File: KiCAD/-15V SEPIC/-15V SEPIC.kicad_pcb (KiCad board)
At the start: 4 copper layers, 33.8 x 28.9 mm, 16 parts, among them U1 LT3579

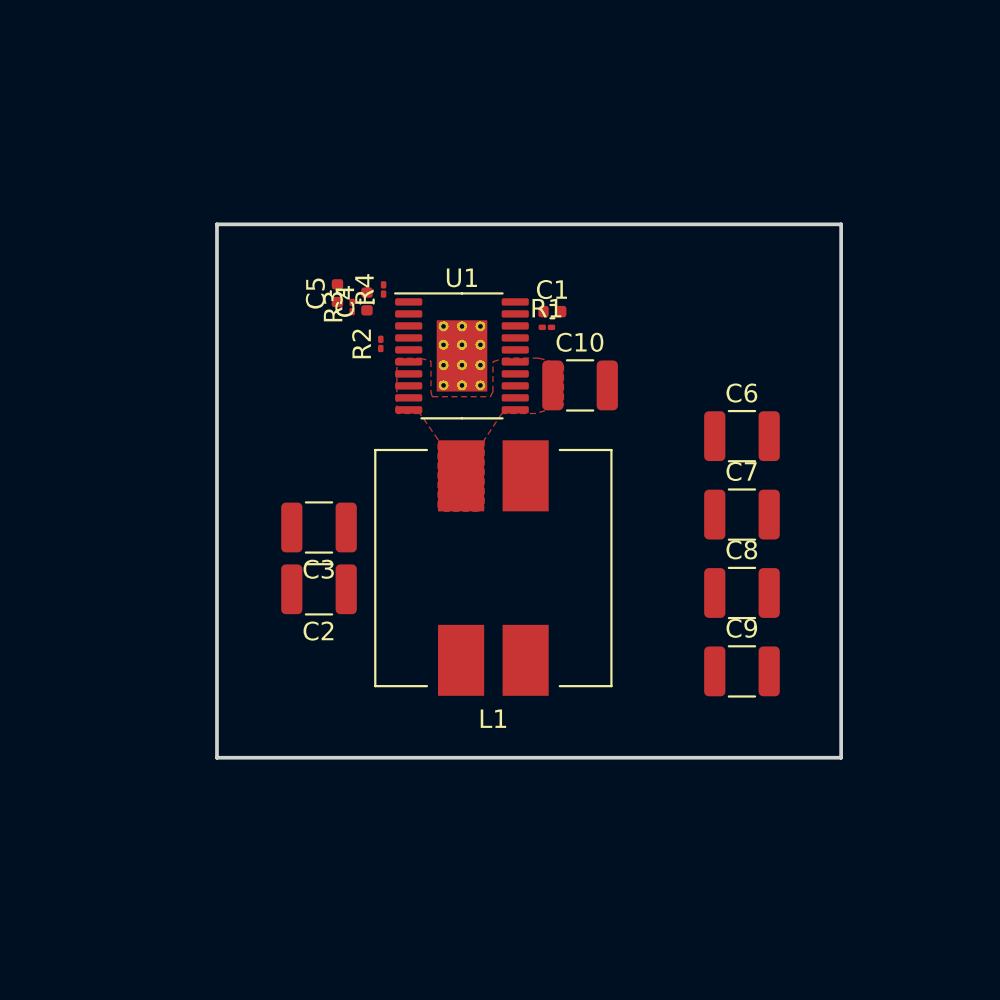
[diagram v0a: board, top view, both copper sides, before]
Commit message: work on speic schematic and PCB
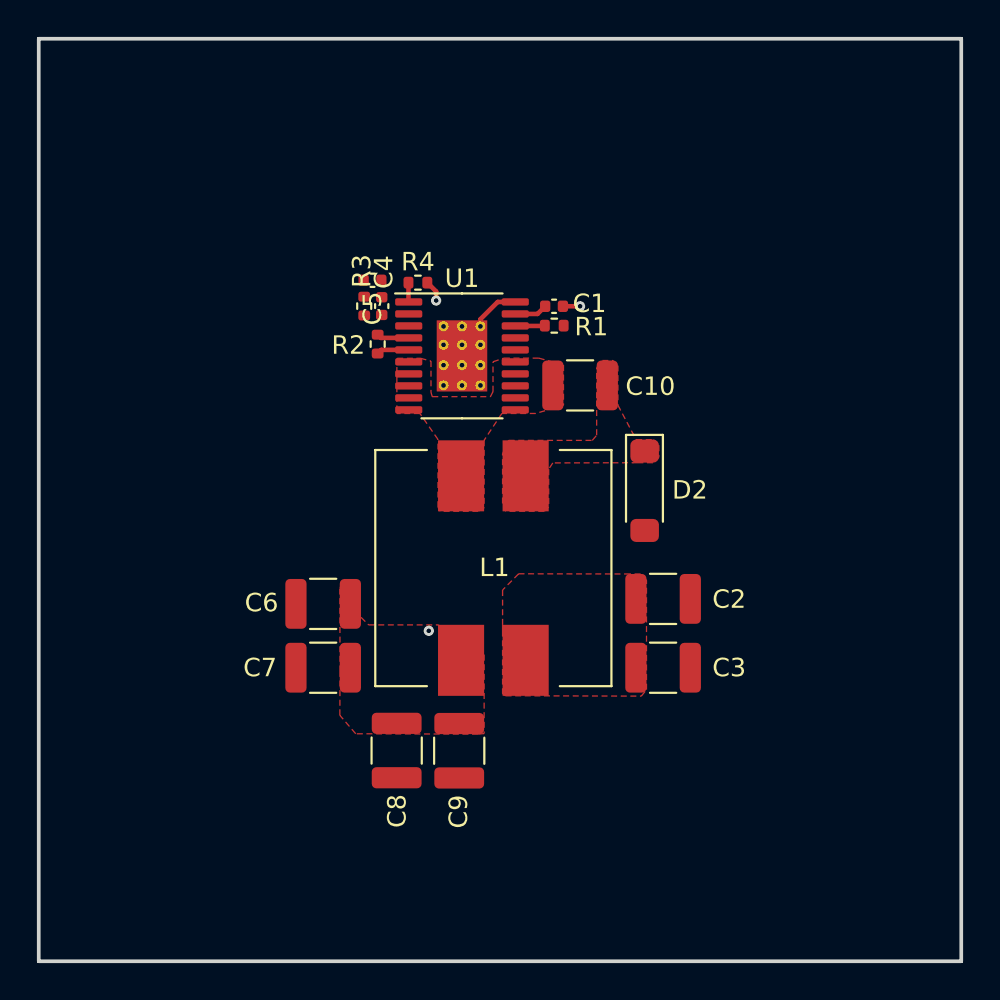
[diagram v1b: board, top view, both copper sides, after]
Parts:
- added D2: VSSAF5L45, footprints:DO-221AC, F.Cu at (73.4, 71.4)
- R1, R2, R3, R4: footprint Resistor_SMD:R_01005_0402Metric -> Resistor_SMD:R_0402_1005Metric
- moved C6 24.5 mm to (56.0, 77.5), turned to 180 degrees
- moved C7 24.2 mm to (56.0, 81.0), turned to 180 degrees
- moved C8 20.6 mm to (60.0, 85.5), turned to -90 degrees
- moved C3 20.1 mm to (74.4, 81.0), turned to 0 degrees
- moved C2 18.7 mm to (74.4, 77.3), turned to 0 degrees
- moved C9 15.9 mm to (63.4, 85.5), turned to -90 degrees
- moved C5 2.02 mm to (58.6, 60.0), turned to 0 degrees
- moved R4 1.90 mm to (61.1, 60.1), turned to 0 degrees
- moved C4 0.84 mm to (59.1, 61.4)
- moved R3 0.65 mm to (58.2, 61.4)
- moved R1 0.41 mm to (68.5, 62.5)
- moved C1 0.30 mm to (68.5, 61.4)
- moved R2 0.17 mm to (58.9, 63.5)
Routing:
- net -15V: track 0.00 -> 20.4 mm, vias 0 -> 2
- net GND: track 0.00 -> 3.59 mm, vias 0 -> 1
- net Net-(U1-SS): track 0.00 -> 1.79 mm
- net Vin (12V - 15V): track 0.00 -> 1.76 mm
- net Net-(U1-~{FAULT}): track 0.00 -> 1.75 mm
- net Net-(U1-RT): track 0.00 -> 1.61 mm
- net Net-(U1-FB): track 0.00 -> 1.05 mm
- added copper zone on F.Cu, net -15V
- added copper zone on F.Cu, net GND
- added copper zone on In1.Cu, net GND
- added copper zone on F.Cu, net Vin (12V - 15V)
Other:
- board size 33.8 x 28.9 mm -> 50 x 50 mm

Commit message: update PCB
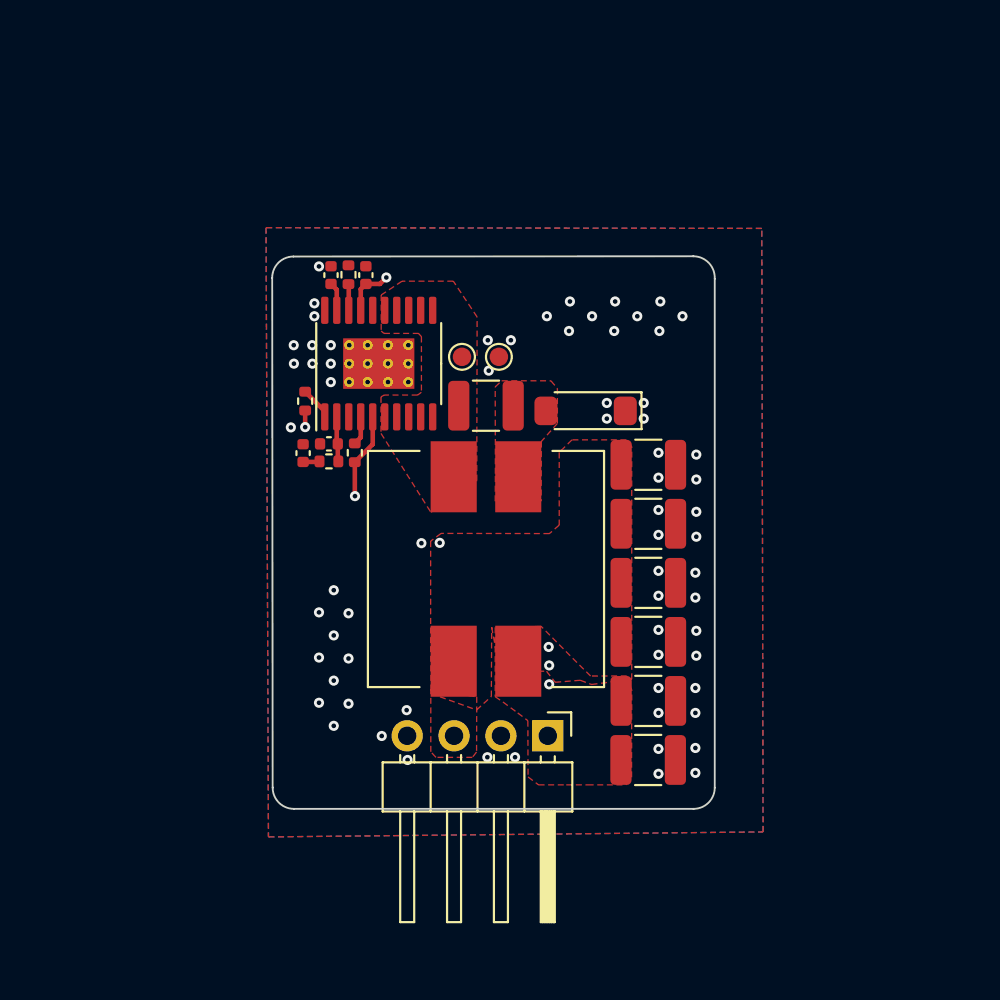
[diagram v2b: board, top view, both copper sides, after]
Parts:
- added C11: 100n, Capacitor_SMD:C_0402_1005Metric, F.Cu at (58.3, 59.7)
- added J1: Conn_01x04_Pin, Connector_PinHeader_2.54mm:PinHeader_1x04_P2.54mm_Horizontal, F.Cu at (68.2, 84.7)
- added TP3: TestPoint, TestPoint:TestPoint_Pad_D1.0mm, F.Cu at (63.5, 64.2)
- added TP5: TestPoint, TestPoint:TestPoint_Pad_D1.0mm, F.Cu at (65.5, 64.2)
- moved C9 18.6 mm to (73.6, 70.0), turned to 0 degrees
- moved C8 18.4 mm to (73.6, 73.2), turned to 0 degrees
- moved C7 18.2 mm to (73.6, 76.4), turned to 0 degrees
- moved C6 17.7 mm to (73.6, 79.6), turned to 0 degrees
- moved C1 12.2 mm to (56.4, 59.7), turned to 90 degrees
- moved R1 11.5 mm to (57.3, 59.7), turned to 90 degrees
- moved C5 10.1 mm to (54.9, 69.4), turned to 90 degrees
- moved R4 8.86 mm to (55.0, 66.5), turned to -90 degrees
- moved R3 8.63 mm to (56.3, 69.8), turned to 180 degrees
- moved C4 8.00 mm to (56.3, 68.9), turned to 180 degrees
- moved R2 6.02 mm to (57.7, 69.3)
- moved C2 5.59 mm to (73.6, 82.8)
- moved D2 5.38 mm to (70.2, 67.1), turned to 180 degrees
- moved C10 5.22 mm to (64.8, 66.8)
- moved C3 5.07 mm to (73.6, 86.0)
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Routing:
- net Vin (12V - 15V): track 1.76 -> 22.3 mm, vias 0 -> 5
- net -15V: track 20.4 -> 12.0 mm
- net GND: track 3.59 -> 0.03 mm, vias 1 -> 68
- net Net-(U1-VC): track 0.00 -> 2.45 mm
- net Net-(C5-Pad1): track 0.00 -> 0.90 mm
- net Net-(U1-FB): track 1.05 -> 1.81 mm
- added copper zone on B.Cu, net GND
- added copper zone on In2.Cu, net GND
- added copper zone on F.Cu, net Net-(D2-A)
- added copper zone on In2.Cu, net Vin (12V - 15V)
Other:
- board size 50 x 50 mm -> 24 x 30 mm
